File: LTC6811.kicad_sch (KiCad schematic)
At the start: 2 parts, among them J1 Conn_01x13, U1 LTC6811-1

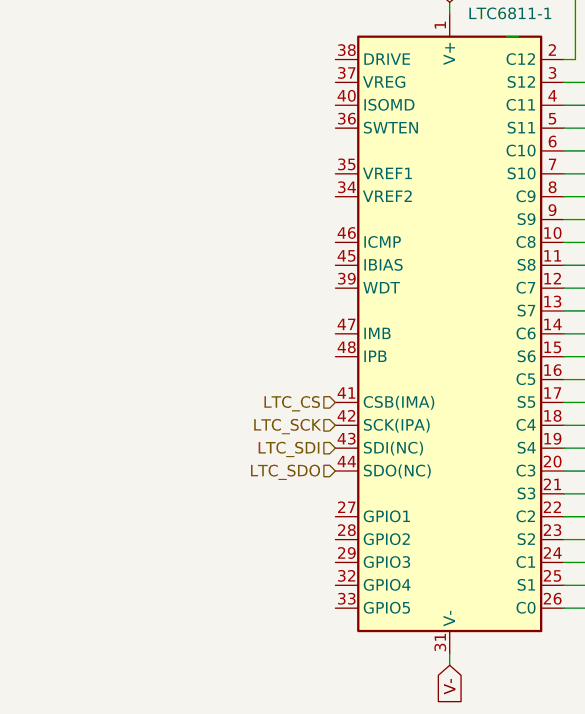
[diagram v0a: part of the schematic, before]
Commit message: update
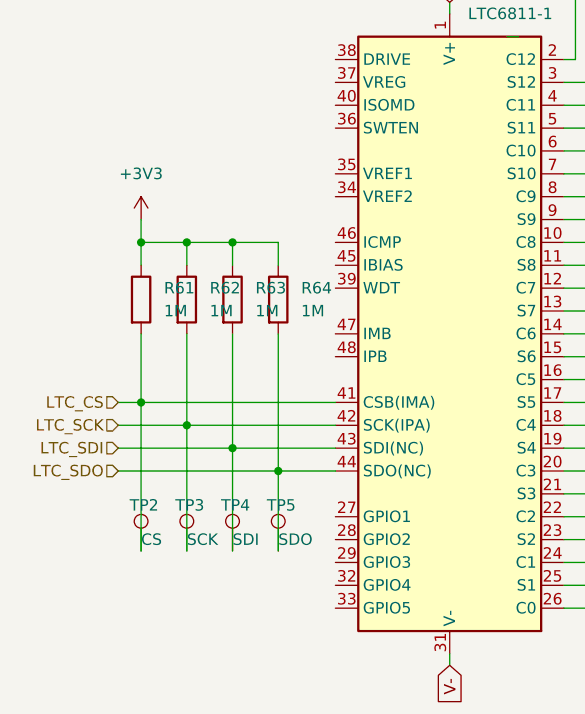
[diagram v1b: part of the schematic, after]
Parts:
- added R61, R62, R63, R64: 1M, symbol Device:R
- added TP2: CS, TestPoint:TestPoint_Pad_D1.5mm, symbol Connector:TestPoint
- added TP3: SCK, TestPoint:TestPoint_Pad_D1.5mm, symbol Connector:TestPoint
- added TP4: SDI, TestPoint:TestPoint_Pad_D1.5mm, symbol Connector:TestPoint
- added TP5: SDO, TestPoint:TestPoint_Pad_D1.5mm, symbol Connector:TestPoint
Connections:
- net LTC_CS: now also R61.2, TP2.1
- net LTC_SCK: now also R62.2, TP3.1
- net LTC_SDI: now also R63.2, TP4.1
- net LTC_SDO: now also R64.2, TP5.1
- new net +3V3: R61.1, R62.1, R63.1, R64.1
